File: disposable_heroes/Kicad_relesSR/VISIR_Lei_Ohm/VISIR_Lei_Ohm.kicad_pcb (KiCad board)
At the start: 2 copper layers, 96 x 90.5 mm, 32 parts, among them J1 Raspberry PI5, J10 Amperimetro+, J11 Amperimetro-, J2 Power Sources, J3 PI_config, J4 Voltimetro+, J5 Ext_OUT_PI, J6 Ext_OUT_PI, J7 Ext_OUT_PI, J8 Ext_OUT_PI, J9 Voltimetro-, K1 3572-1220-123, K2 3572-1220-123, K3 3572-1220-123, K4 3570-1331-123, K5 3570-1331-123, K6 3570-1331-123, K7 3570-1331-123, K8 3570-1331-123, U1 74HC595N_112, U2 ULN2003, U3 ULN2003

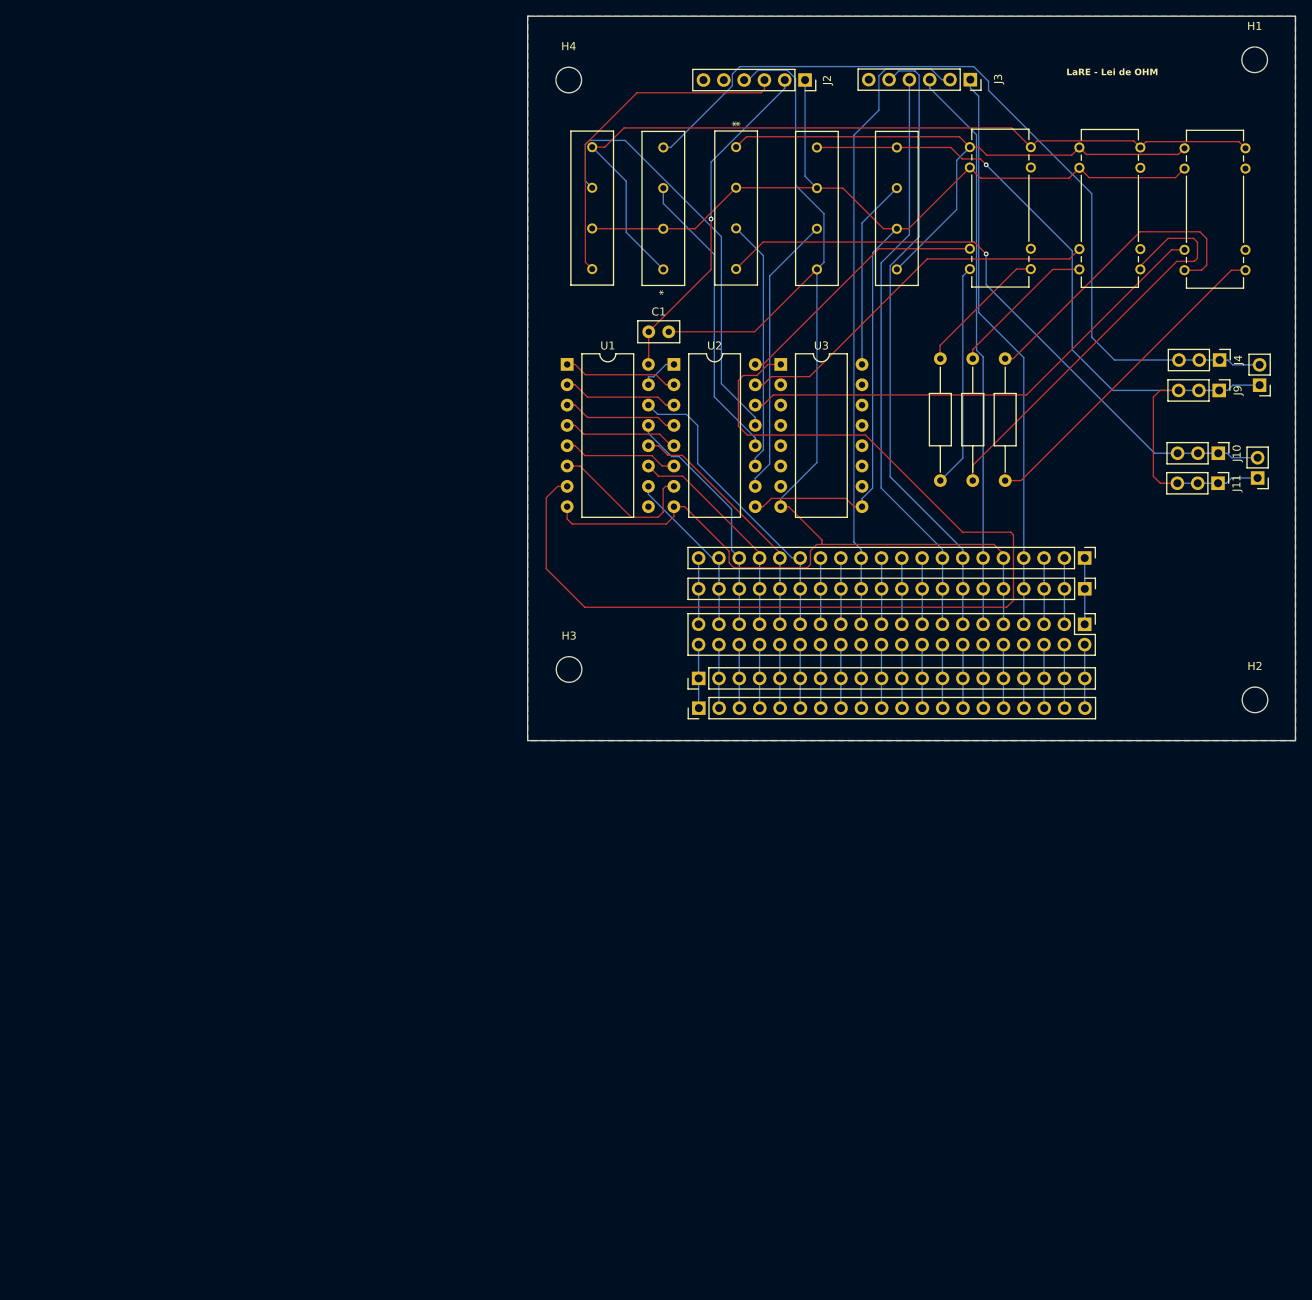
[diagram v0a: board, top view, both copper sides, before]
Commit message: update kicad files
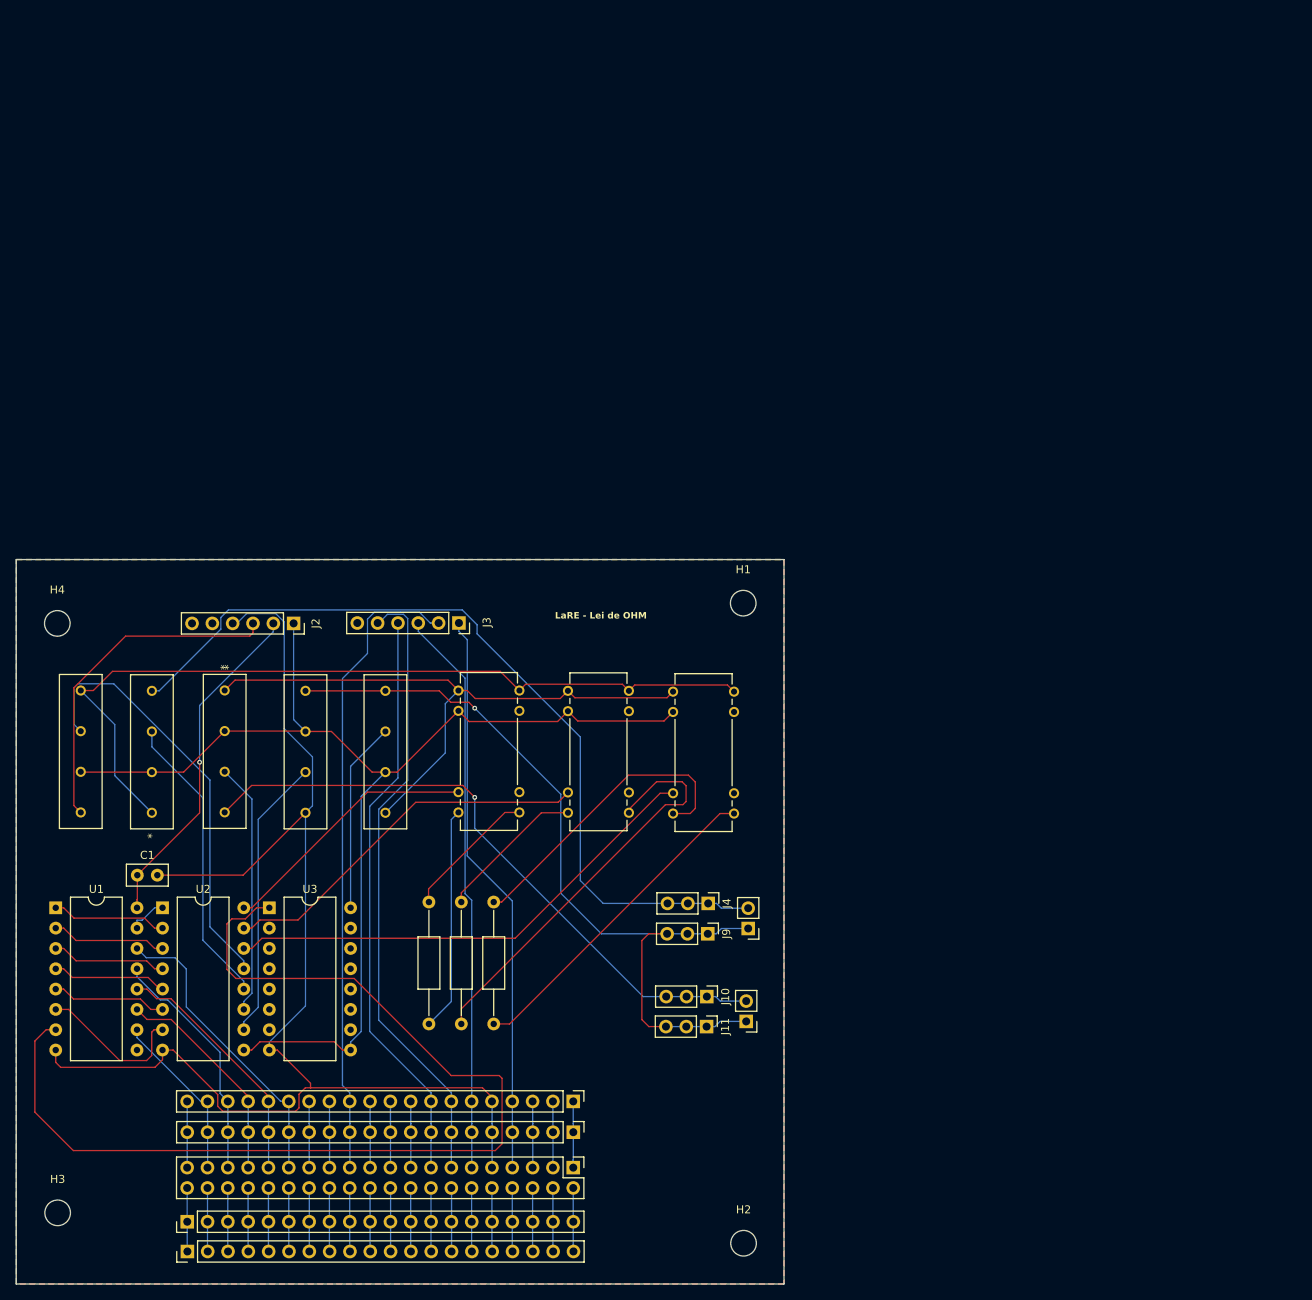
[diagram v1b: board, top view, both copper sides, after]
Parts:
- moved H3 93.3 mm to (61.9, 179.8)
- moved J5 93.3 mm to (78.1, 180.9)
- moved K3 93.3 mm to (138.8, 114.7)
- moved H4 93.3 mm to (61.8, 106.2)
- moved J10 93.3 mm to (143.0, 152.8)
- moved J11 93.3 mm to (143.0, 156.6)
- moved J2 93.3 mm to (91.4, 106.2)
- moved K1 93.3 mm to (112.0, 114.5)
- moved C1 93.3 mm to (71.8, 137.6)
- moved H1 93.3 mm to (147.6, 103.6)
- moved H2 93.3 mm to (147.6, 183.6)
- moved J1 93.3 mm to (126.3, 174.2)
- moved J4 93.3 mm to (143.2, 141.2)
- moved J6 93.3 mm to (78.1, 184.7)
- moved J7 93.3 mm to (126.3, 169.8)
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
